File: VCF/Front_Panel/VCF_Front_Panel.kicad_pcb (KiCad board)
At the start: 2 copper layers, 40.1 x 128.5 mm, 8 parts

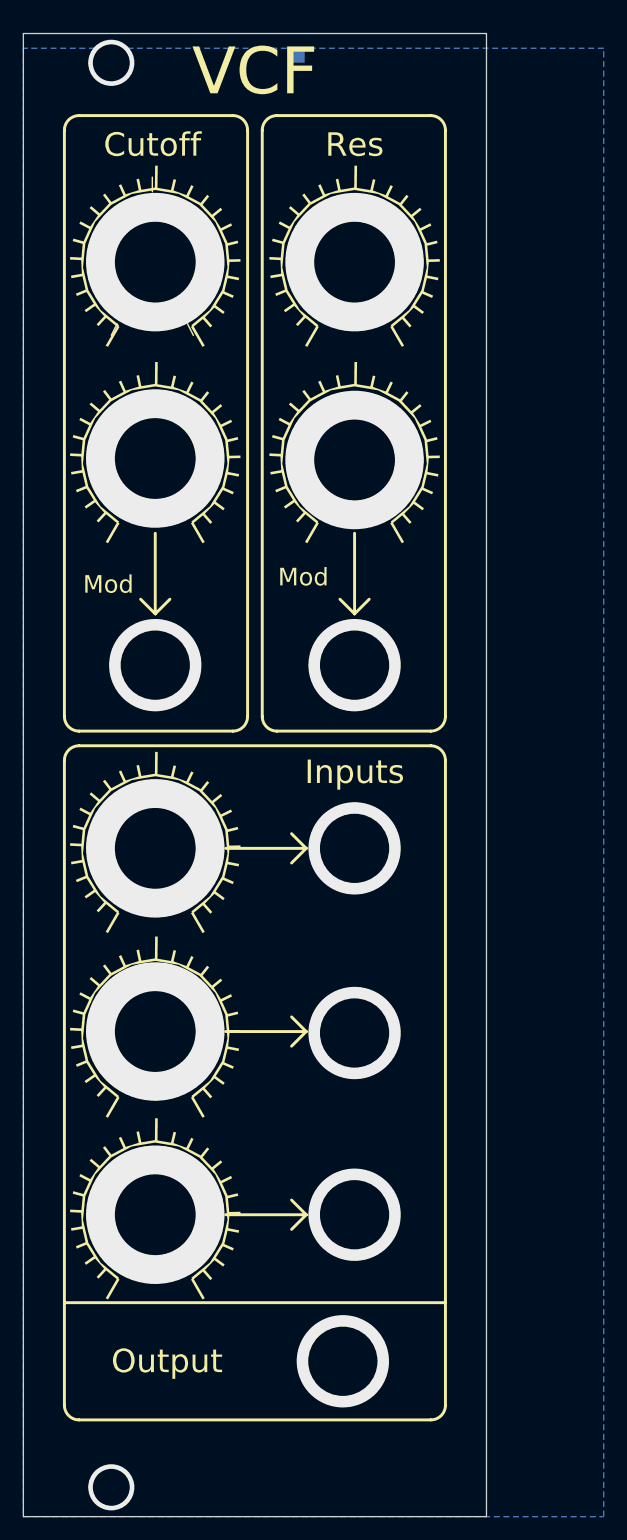
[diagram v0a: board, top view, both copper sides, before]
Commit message: Clean up VCF boards
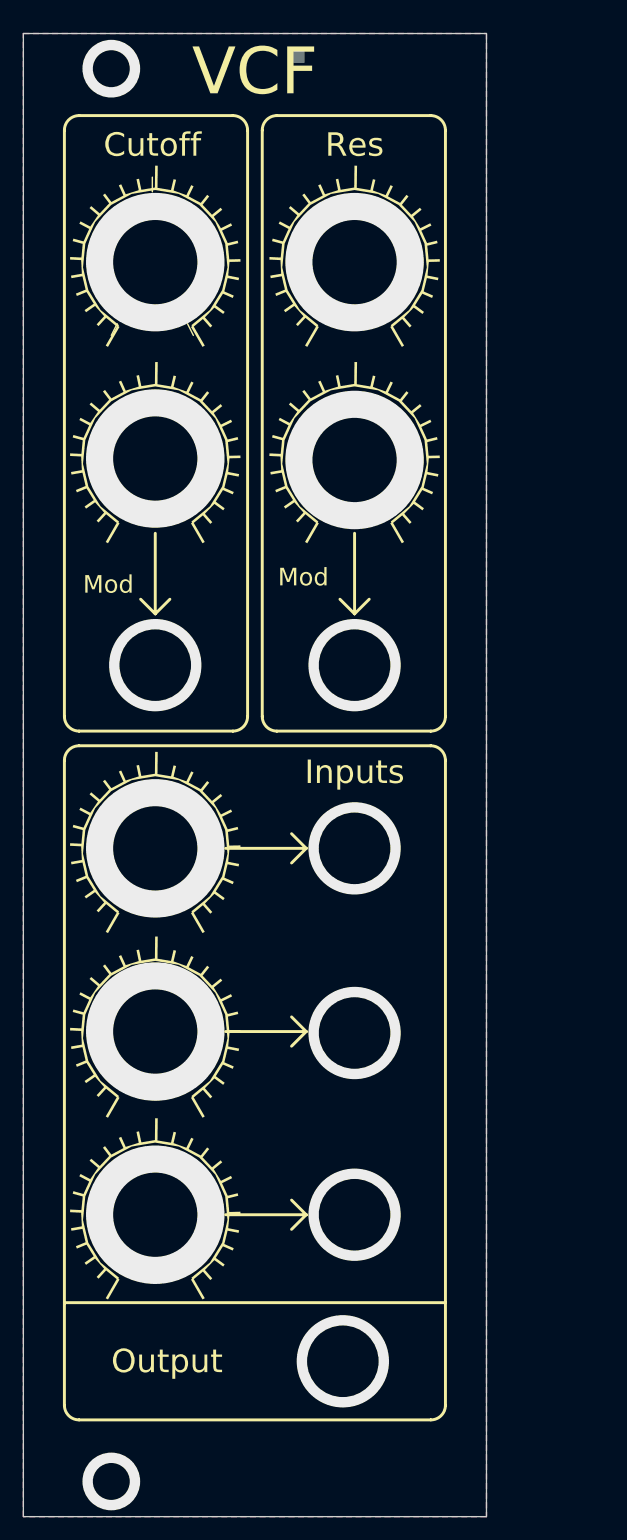
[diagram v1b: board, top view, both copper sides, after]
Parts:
- added REF**: OSHW-Logo2_7.3x6mm_SilkScreen, Symbol:OSHW-Logo2_7.3x6mm_SilkScreen, B.Cu at (92.5, 47.8)
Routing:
- added copper zone on F.Cu, net GND
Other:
- board text added: "WH"
